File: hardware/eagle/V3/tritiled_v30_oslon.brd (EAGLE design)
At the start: 22.9 x 22.9 mm, 12 parts, among them IC1 PIC12LF1571, IC2 74LVC1G123, Q1 IRLML6244, Q2 DMG2305UX

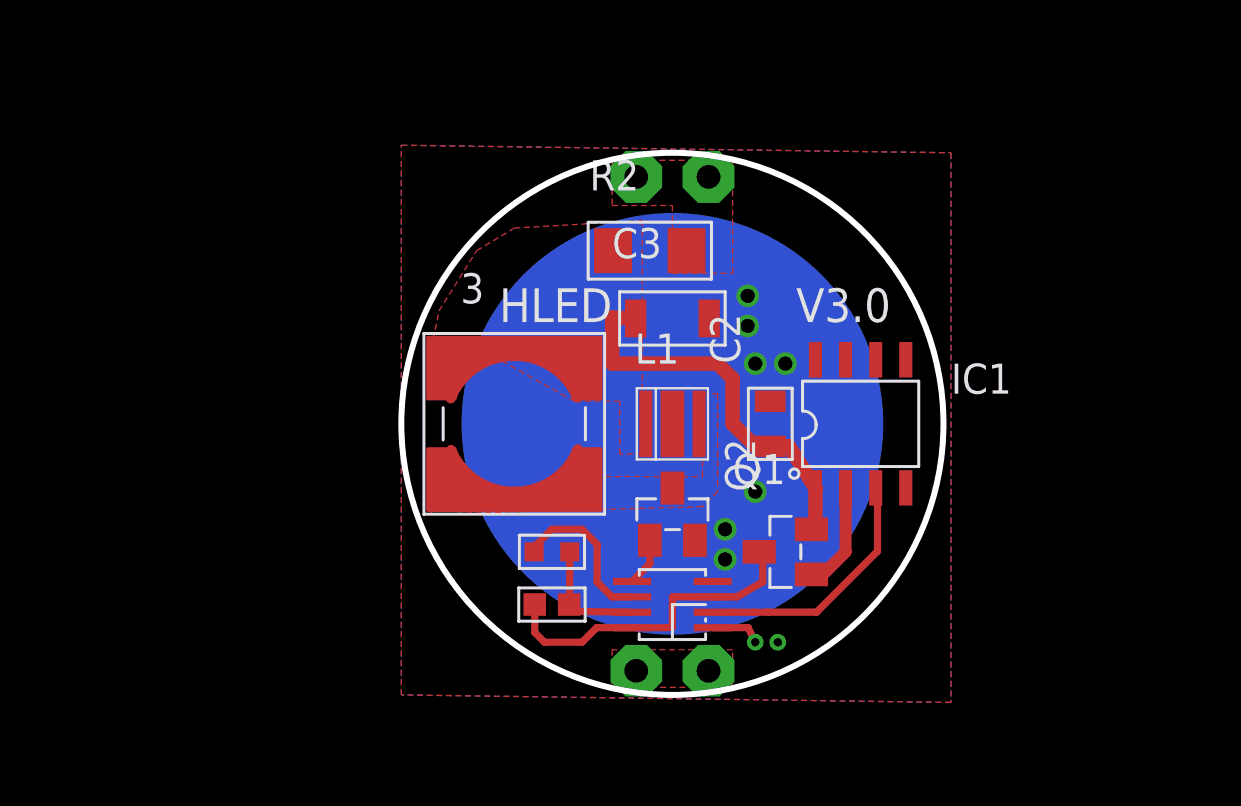
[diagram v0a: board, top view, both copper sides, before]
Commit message: updated files for initial V3.0 release
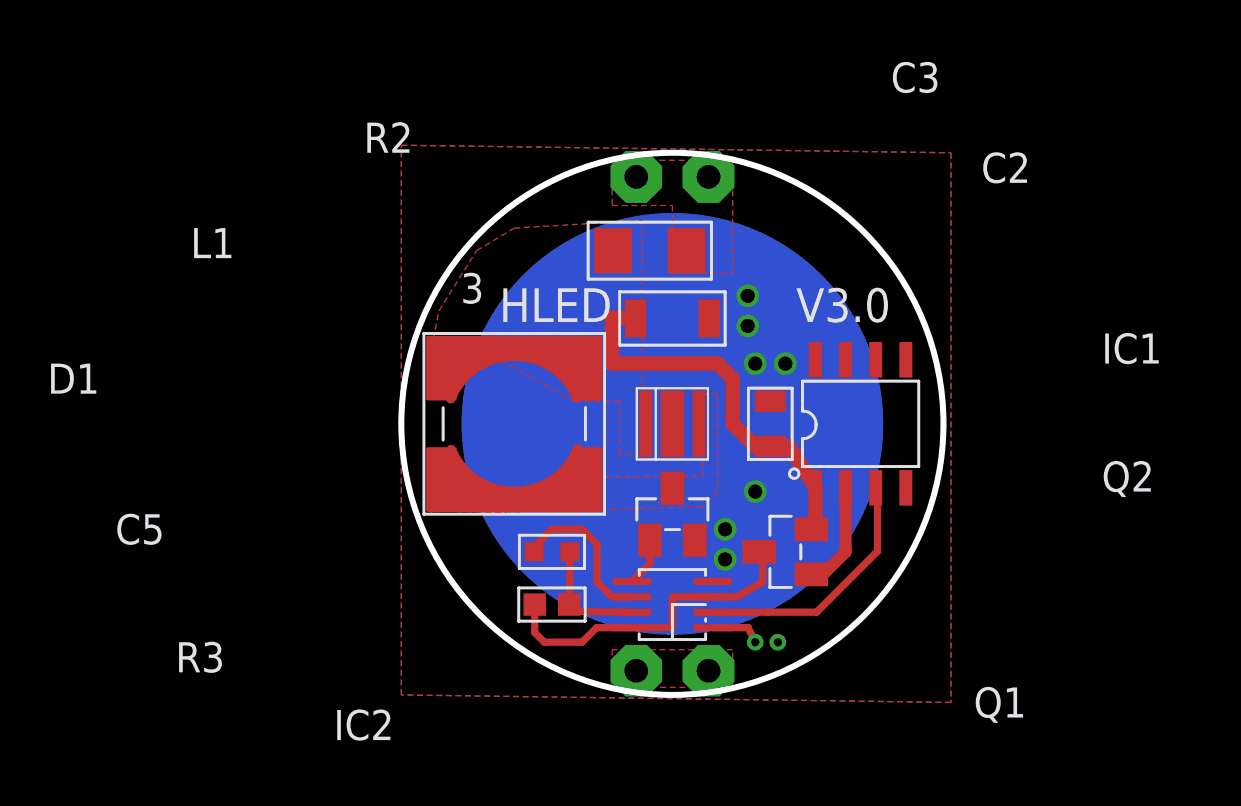
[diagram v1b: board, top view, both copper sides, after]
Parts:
- C2: value 100n -> 1u
- D1: value OSLON Signal -> OSLON S.V.
- R3: value 10k -> 51k
- renumbered U$1 to D1
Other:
- board text added: "(cathode left)"
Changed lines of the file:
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@@
 <?xml version="1.0" encoding="utf-8"?>
 <!DOCTYPE eagle SYSTEM "eagle.dtd">
-<eagle version="8.2.2">
+<eagle version="8.5.0">
 <drawing>
 <settings>
 <setting alwaysvectorfont="yes"/>
+<setting keepoldvectorfont="yes"/>
 <setting verticaltext="up"/>
 </settings>
@@
 <layers>
 <layer number="1" name="Top" color="4" fill="1" visible="yes" active="yes"/>
+<layer number="2" name="Route2" color="1" fill="3" visible="no" active="no"/>
+<layer number="15" name="Route15" color="4" fill="6" visible="no" active="no"/>
 <layer number="16" name="Bottom" color="1" fill="1" visible="yes" active="yes"/>
 <layer number="17" name="Pads" color="2" fill="1" visible="yes" active="yes"/>
@@
 <layer number="23" name="tOrigins" color="15" fill="1" visible="yes" active="yes"/>
 <layer number="24" name="bOrigins" color="15" fill="1" visible="yes" active="yes"/>
-<layer number="25" name="tNames" color="7" fill="1" visible="no" active="yes"/>
+<layer number="25" name="tNames" color="7" fill="1" visible="yes" active="yes"/>
 <layer number="26" name="bNames" color="7" fill="1" visible="no" active="yes"/>
-<layer number="27" name="tValues" color="7" fill="1" visible="no" active="yes"/>
+<layer number="27" name="tValues" color="7" fill="1" visible="yes" active="yes"/>
 <layer number="28" name="bValues" color="7" fill="1" visible="no" active="yes"/>
 <layer number="29" name="tStop" color="7" fill="3" visible="no" active="yes"/>
@@
 <text x="20.6375" y="17.145" size="1.4224" layer="21" font="fixed" ratio="13" rot="R180">V3.0</text>
 <text x="3.4925" y="17.78" size="1.27" layer="21" font="fixed" ratio="13" rot="R180">3</text>
+<dimension x1="10.4775" y1="18.7325" x2="1.27" y2="22.225" x3="1.27" y3="22.225" textsize="1.778" layer="51" dtype="leader"/>
+<dimension x1="11.43" y1="15.875" x2="19.3675" y2="24.4475" x3="19.3675" y3="24.4475" textsize="1.778" layer="51" dtype="leader"/>
+<dimension x1="15.5575" y1="11.43" x2="23.8125" y2="20.6375" x3="23.8125" y3="20.6375" textsize="1.778" layer="51" dtype="leader"/>
+<dimension x1="19.3675" y1="11.43" x2="25.0825" y2="13.335" x3="25.0825" y3="13.335" textsize="1.778" layer="51" dtype="leader"/>
+<dimension x1="16.1925" y1="6.0325" x2="25.0825" y2="7.9375" x3="25.0825" y3="7.9375" textsize="1.778" layer="51" dtype="leader"/>
+<dimension x1="11.43" y1="7.62" x2="20.32" y2="-1.27" x3="20.32" y3="-1.27" textsize="1.778" layer="51" dtype="leader"/>
+<dimension x1="11.43" y1="3.81" x2="0.9525" y2="-1.905" x3="0.9525" y3="-1.905" textsize="1.778" layer="51" dtype="leader"/>
+<dimension x1="6.35" y1="3.81" x2="-6.985" y2="0.635" x3="-6.985" y3="0.635" textsize="1.778" layer="51" dtype="leader"/>
+<dimension x1="6.35" y1="6.0325" x2="-9.525" y2="6.0325" x3="-9.525" y3="6.0325" textsize="1.778" layer="51" dtype="leader"/>
+<dimension x1="4.7625" y1="11.43" x2="-6.6675" y2="17.78" x3="-6.6675" y3="17.78" textsize="1.778" layer="51" dtype="leader"/>
+<dimension x1="11.43" y1="11.43" x2="-3.4925" y2="9.2075" x3="-3.4925" y3="9.2075" textsize="1.778" layer="51" dtype="leader"/>
+<text x="-19.3675" y="8.89" size="1.4224" layer="51">(cathode left)</text>
 </plain>
 <attributes>
@@
 <param name="dpMaxLengthDifference" value="10mm"/>
 <param name="dpGapFactor" value="2.5"/>
-<param name="checkGrid" value="0"/>
 <param name="checkAngle" value="1"/>
 <param name="checkFont" value="1"/>
 <param name="checkRestrict" value="1"/>
+<param name="checkStop" value="0"/>
+<param name="checkValues" value="0"/>
 <param name="useDiameter" value="13"/>
 <param name="maxErrors" value="50"/>
@@
 </autorouter>
 <elements>
-<element name="C2" library="tritiled" package="0805" value="100n" x="15.5575" y="11.43" rot="R90"/>
-<element name="IC1" library="tritiled" package="SOIC8" value="PIC12LF1571" x="19.3675" y="11.43"/>
-<element name="Q1" library="tritiled" package="SOT-23" value="IRLML6244" x="11.43" y="7.62"/>
-<element name="U$1" library="tritiled" package="OSLON_3030_LED" value="OSLON Signal" x="11.43" y="11.43" rot="R180"/>
+<element name="C2" library="tritiled" package="0805" value="1u" x="15.5575" y="11.43" smashed="yes" rot="R90">
+<attribute name="NAME" x="24.4475" y="21.59" size="1.27" layer="25"/>
+<attribute name="VALUE" x="24.13" y="19.3675" size="1.27" layer="27"/>
+</element>
+<element name="IC1" library="tritiled" package="SOIC8" value="PIC12LF1571" x="19.3675" y="11.43" smashed="yes">
+<attribute name="NAME" x="29.5275" y="13.97" size="1.27" layer="25"/>
+<attribute name="VALUE" x="25.7175" y="12.065" size="1.27" layer="27"/>
+</element>
+<element name="Q1" library="tritiled" package="SOT-23" value="IRLML6244" x="11.43" y="7.62" smashed="yes">
+<attribute name="NAME" x="24.13" y="-0.9525" size="1.27" layer="25"/>
+<attribute name="VALUE" x="20.6375" y="-2.8575" size="1.27" layer="27"/>
+</element>
+<element name="D1" library="tritiled" package="OSLON_3030_LED" value="OSLON S.V." x="11.43" y="11.43" smashed="yes" rot="R180">
+<attribute name="NAME" x="-14.9225" y="12.7" size="1.27" layer="25"/>
+<attribute name="VALUE" x="-17.78" y="10.795" size="1.27" layer="27"/>
+</element>
 <element name="B1" library="tritiled" package="CR2032_BAT-HLD-001-THM" value="BAT-HLD-001-THM_CR2032" x="11.43" y="11.43" rot="MR270"/>
-<element name="L1" library="tritiled" package="SRR6028_INDUCTOR" value="1m" x="4.7625" y="11.43"/>
-<element name="R2" library="tritiled" package="R1206" value="100" x="10.4775" y="18.7325"/>
-<element name="C3" library="tritiled" package="1206" value="10u" x="11.43" y="15.875"/>
-<element name="IC2" library="tritiled" package="SM8" value="74LVC1G123" x="11.43" y="3.81" rot="R90"/>
-<element name="R3" library="tritiled" package="R0603" value="10k" x="6.35" y="3.81" rot="R180"/>
-<element name="C5" library="tritiled" package="C0603" value="100p" x="6.35" y="6.0325" rot="R180"/>
-<element name="Q2" library="tritiled" package="SOT-23" value="DMG2305UX" x="16.1925" y="6.0325" rot="R90"/>
+<element name="L1" library="tritiled" package="SRR6028_INDUCTOR" value="1m" x="4.7625" y="11.43" smashed="yes">
+<attribute name="NAME" x="-8.89" y="18.415" size="1.27" layer="25"/>
+<attribute name="VALUE" x="-9.2075" y="16.1925" size="1.27" layer="27"/>
+</element>
+<element name="R2" library="tritiled" package="R1206" value="100" x="10.4775" y="18.7325" smashed="yes">
+<attribute name="NAME" x="-1.5875" y="22.86" size="1.27" layer="25"/>
+<attribute name="VALUE" x="-2.2225" y="20.6375" size="1.27" layer="27"/>
+</element>
+<element name="C3" library="tritiled" package="1206" value="10u" x="11.43" y="15.875" smashed="yes">
+<attribute name="NAME" x="20.6375" y="25.4" size="1.27" layer="25"/>
+<attribute name="VALUE" x="20.0025" y="23.495" size="1.27" layer="27"/>
+</element>
+<element name="IC2" library="tritiled" package="SM8" value="74LVC1G123" x="11.43" y="3.81" smashed="yes" rot="R90">
+<attribute name="NAME" x="-2.8575" y="-1.905" size="1.27" layer="25"/>
+<attribute name="VALUE" x="-6.0325" y="-4.1275" size="1.27" layer="27"/>
+</element>
+<element name="R3" library="tritiled" package="R0603" value="51k" x="6.35" y="3.81" smashed="yes" rot="R180">
+<attribute name="NAME" x="-9.525" y="0.9525" size="1.27" layer="25"/>
+<attribute name="VALUE" x="-10.16" y="-1.27" size="1.27" layer="27"/>
+</element>
+<element name="C5" library="tritiled" package="C0603" value="100p" x="6.35" y="6.0325" smashed="yes" rot="R180">
+<attribute name="NAME" x="-12.065" y="6.35" size="1.27" layer="25"/>
+<attribute name="VALUE" x="-13.0175" y="4.1275" size="1.27" layer="27"/>
+</element>
+<element name="Q2" library="tritiled" package="SOT-23" value="DMG2305UX" x="16.1925" y="6.0325" smashed="yes" rot="R90">
+<attribute name="NAME" x="29.5275" y="8.5725" size="1.27" layer="25"/>
+<attribute name="VALUE" x="25.7175" y="6.6675" size="1.27" layer="27"/>
+</element>
 </elements>
 <signals>
 <signal name="+3.6V">
 <contactref element="L1" pad="P$1"/>
-<contactref element="U$1" pad="C"/>
+<contactref element="D1" pad="C"/>
 <contactref element="IC1" pad="1"/>
 <contactref element="C2" pad="P$1"/>
@@
 <via x="15.875" y="2.2225" extent="1-16" drill="0.35"/>
 </signal>
-<signal name="N$9">
+<signal name="N$9" airwireshidden="yes">
 <contactref element="B1" pad="+V@1"/>
 <contactref element="R2" pad="P$2"/>
@@
 <contactref element="L1" pad="P$2"/>
 <contactref element="Q1" pad="3"/>
-<contactref element="U$1" pad="A"/>
+<contactref element="D1" pad="A"/>
 <polygon width="0.254" layer="1" orphans="yes" thermals="no">
 <vertex x="12.7" y="12.7"/>
